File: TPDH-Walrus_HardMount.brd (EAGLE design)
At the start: 12.7 x 42 mm, 30 parts, among them Q2 DMG3404, U1 MS5803-14BA, U2 SN65HVD72DSOIC, U4 MCP9808MSOP, U5 LP39883.3VDBV, U7 TXS0102DQM, U8 NS5A4684S

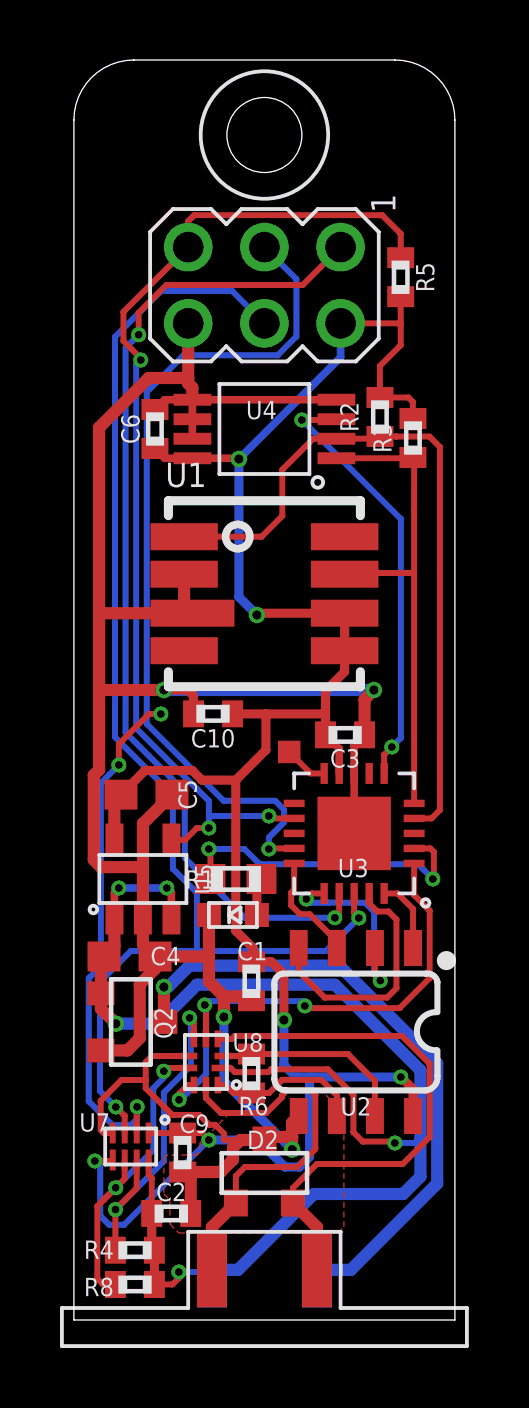
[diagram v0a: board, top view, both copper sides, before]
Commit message: Board cleanup, final DFM for v0.2, added gerbers
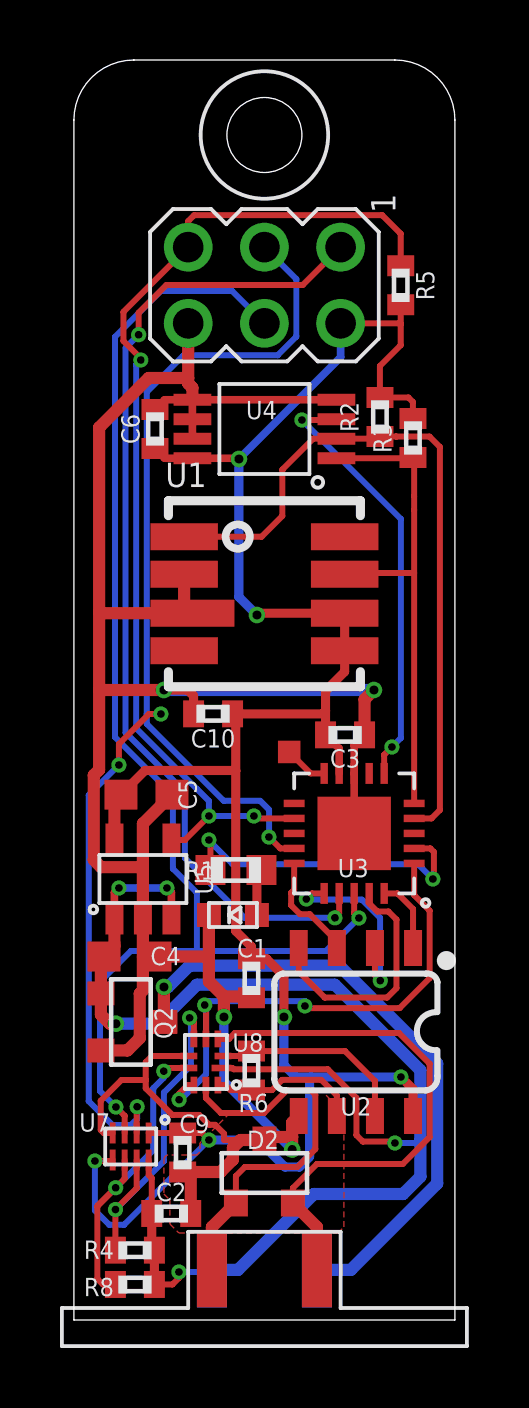
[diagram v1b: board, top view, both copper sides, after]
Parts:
- moved R1 0.30 mm to (5.40, 15.0)
- moved R5 0.27 mm to (10.9, 34.5)
- moved C1 0.10 mm to (5.92, 11.4)
- moved R6 0.10 mm to (5.92, 8.31)
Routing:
- net SCL: track 46.3 -> 45.3 mm
- net +3V3: track 74.7 -> 73.8 mm
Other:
- board text added: "Project-TPDH-Walrus v0.2.0 07-15-2019 Based on TP-Downhole by Schulz, Sandell, Wickert A. Wickert Northern Widget LLC and University of Minnesota"
- board text removed: "Project-TPDH-Walrus v0.1.0 07-15-2019 Based on TP-Downhole by Schulz, Sandell, Wickert A. Wickert Northern Widget LLC and University of Minnesota"
